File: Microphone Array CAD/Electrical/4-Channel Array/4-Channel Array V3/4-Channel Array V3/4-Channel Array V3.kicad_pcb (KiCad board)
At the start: 2 copper layers, 35 x 35 mm, 20 parts, among them J1 Conn_01x05_Pin, U1 74LCX125MTCX

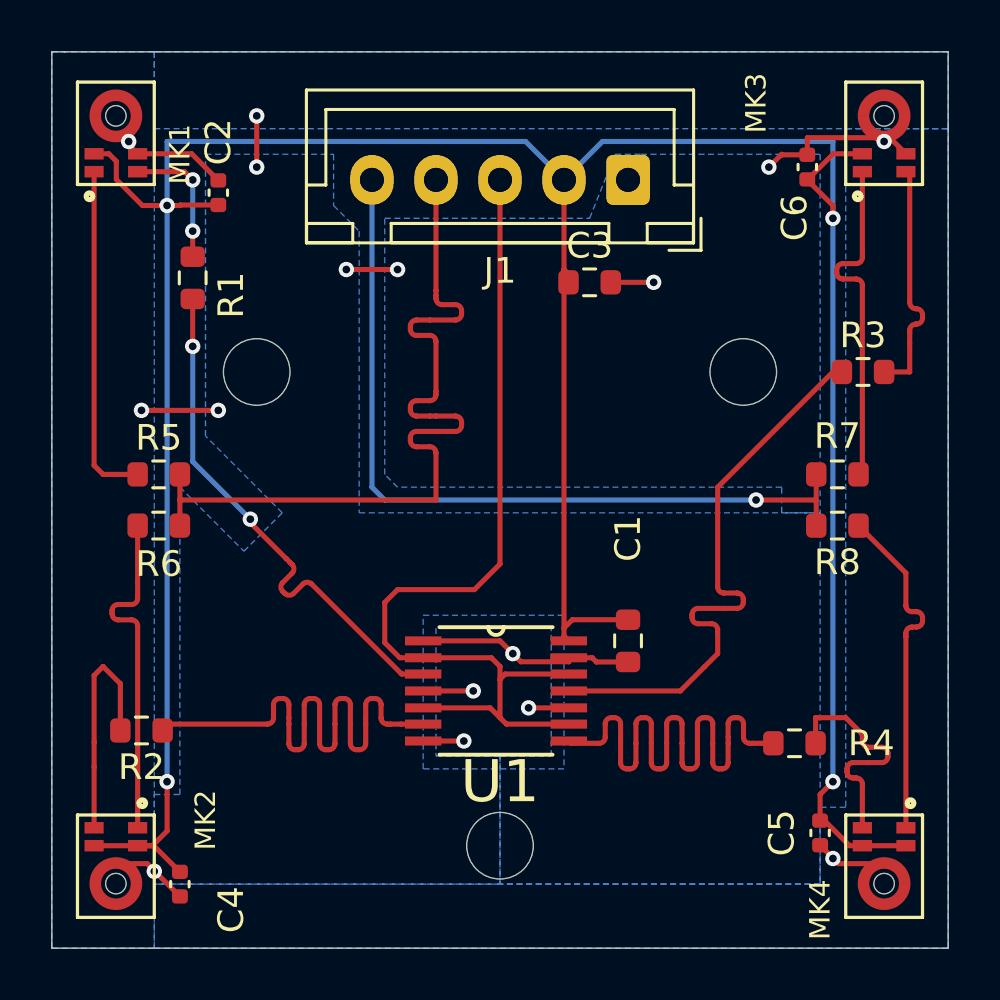
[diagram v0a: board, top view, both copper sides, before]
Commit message: Continued Array Development
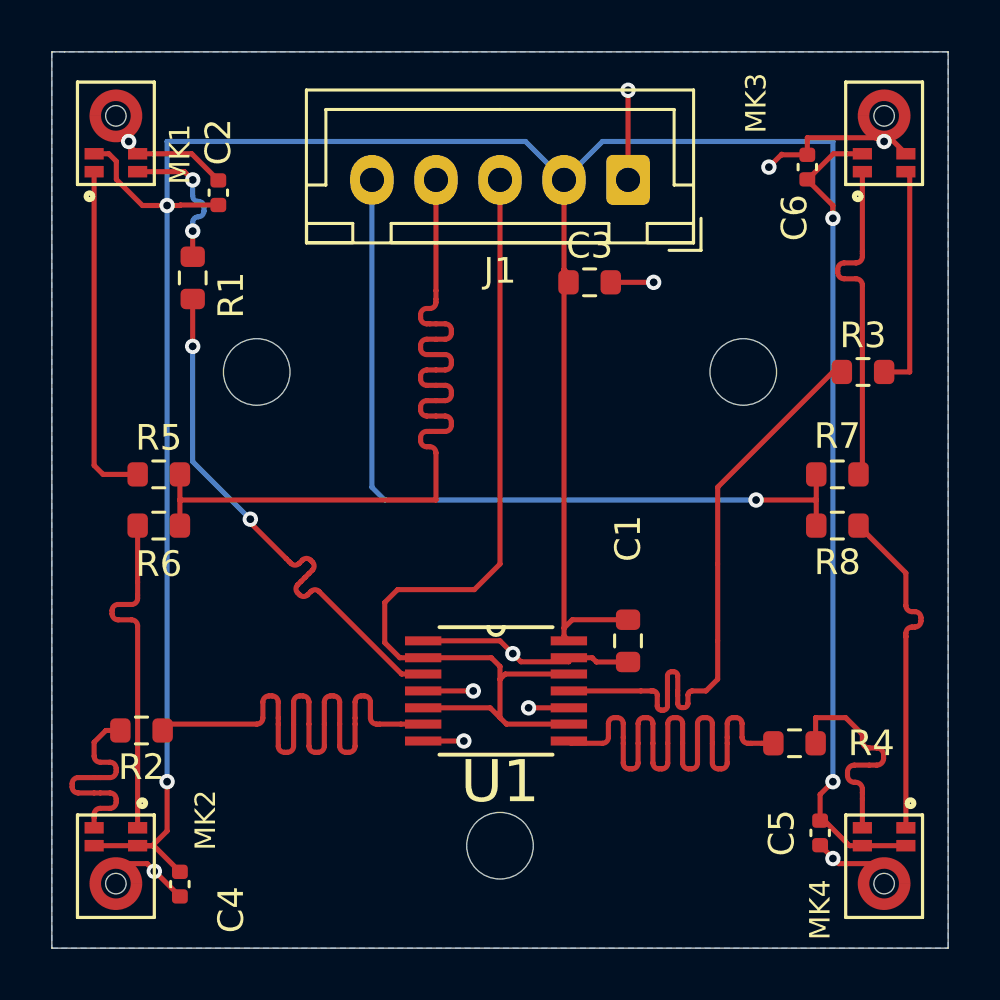
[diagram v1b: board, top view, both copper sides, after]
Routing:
- net Net-(J1-Pin_1): track 39.8 -> 36.3 mm, vias 16 -> 11
- net Net-(U1-O1): track 22.5 -> 23.9 mm
- net Net-(U1-O2): track 23.0 -> 23.9 mm
- net Net-(MK3-CLK): track 9.43 -> 8.88 mm

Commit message: Restructure
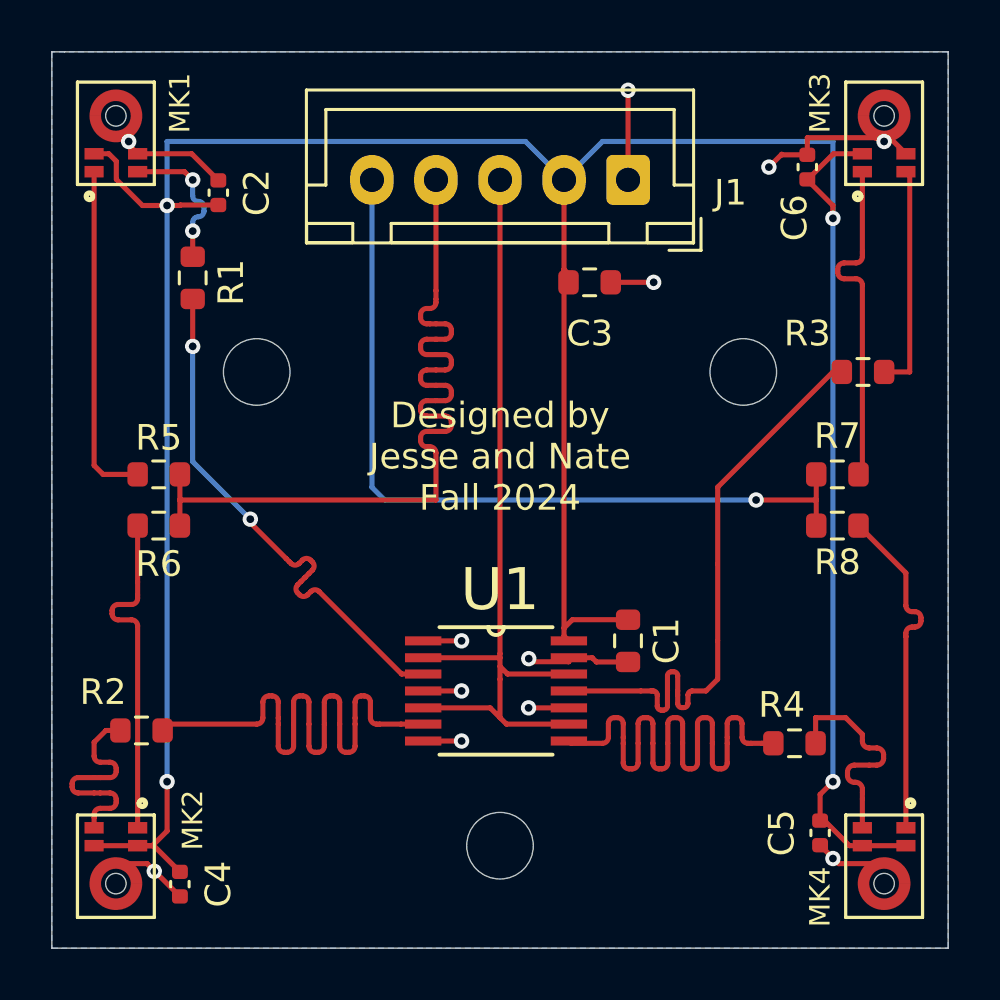
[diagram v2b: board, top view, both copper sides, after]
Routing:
- net Net-(J1-Pin_3): track 37.3 -> 32.8 mm
- net Net-(J1-Pin_1): track 36.3 -> 32.9 mm, vias 11 -> 12
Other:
- board text added: "Designed by Jesse and Nate Fall 2024"
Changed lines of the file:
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@@
 		(tags "connector JST XH vertical")
 		(property "Reference" "J1"
-			(at 5 -3.55 0)
+			(at -4 -0.5 0)
 			(layer "F.SilkS")
 			(effects
@@
 		(tags "resistor")
 		(property "Reference" "R3"
-			(at 0 -1.43 0)
+			(at -2.175 -1.5 0)
 			(layer "F.SilkS")
 			(effects
@@
 		(tags "resistor")
 		(property "Reference" "R1"
-			(at -0.675 1.5 90)
+			(at -0.175 1.5 90)
 			(layer "F.SilkS")
 			(effects
@@
 		(tags "capacitor")
 		(property "Reference" "C2"
-			(at 1.98 0 90)
+			(at 0 1.5 90)
 			(layer "F.SilkS")
 			(effects
@@
 		(tags "resistor")
 		(property "Reference" "C3"
-			(at 0 -1.43 0)
+			(at 0 2 0)
 			(layer "F.SilkS")
 			(effects
@@
 		(at 180 79.3 -90)
 		(property "Reference" "MK4"
-			(at 1.7 2.5 90)
+			(at 1.2 2.5 90)
 			(layer "F.SilkS")
 			(effects
@@
 		(at 150 79.3 -90)
 		(property "Reference" "MK2"
-			(at -1.8 -3.5 90)
+			(at -1.8 -3 90)
 			(layer "F.SilkS")
 			(effects
@@
 		(at 180 50.68 90)
 		(property "Reference" "MK3"
-			(at 1.18 -5 90)
+			(at 1.18 -2.5 90)
 			(layer "F.SilkS")
 			(effects
@@
 		(at 164.8448 72.4558)
 		(property "Reference" "U1"
-			(at 0.1552 3.5442 0)
+			(at 0.1552 -3.9558 0)
 			(layer "F.SilkS")
 			(effects
@@
 		(tags "resistor")
 		(property "Reference" "R2"
-			(at 0 -1.43 0)
+			(at 1.5 1.5 0)
 			(layer "F.SilkS")
 			(effects
@@
 		(tags "resistor")
 		(property "Reference" "C1"
-			(at 4 0 90)
+			(at 0 1.5 90)
 			(layer "F.SilkS")
 			(effects
@@
 		(tags "capacitor")
 		(property "Reference" "C4"
-			(at 1 -2 90)
+			(at 0 -1.5 90)
 			(layer "F.SilkS")
 			(effects
@@
 		(tags "resistor")
 		(property "Reference" "R4"
-			(at 3 0 0)
+			(at -0.5 -1.5 0)
 			(layer "F.SilkS")
 			(effects
@@
 		(at 150 50.68 90)
 		(property "Reference" "MK1"
-			(at -0.82 2.5 90)
+			(at 1.18 2.5 90)
 			(layer "F.SilkS")
 			(effects
@@
 		(layer "Edge.Cuts")
 	)
+	(gr_text "Designed by \nJesse and Nate\nFall 2024"
+		(at 165 65.5 0)
+		(layer "F.SilkS")
+		(effects
+			(font
+				(size 1 1)
+				(thickness 0.1)
+			)
+			(justify bottom)
+		)
+	)
 	(segment
 		(start 149.725 51.48)
@@
 	)
 	(segment
+		(start 166.1162 73.1162)
+		(end 167.6896 73.1162)
+		(width 0.2)
+		(layer "F.Cu")
+		(net 2)
+	)
+	(segment
 		(start 151.5 79.48)
 		(end 151.22 79.2)
@@
 	)
 	(segment
+		(start 163.5 72.4558)
+		(end 162 72.4558)
+		(width 0.2)
+		(layer "F.Cu")
+		(net 2)
+	)
+	(segment
 		(start 168.6008 71.1604)
 		(end 168.7654 71.325)
@@
 	)
 	(segment
-		(start 165.8176 71.3176)
-		(end 167.6824 71.3176)
-		(width 0.2)
-		(layer "F.Cu")
-		(net 2)
-	)
-	(segment
 		(start 151.22 79.2)
 		(end 150 79.2)
@@
 	)
 	(segment
-		(start 167.6824 71.3176)
-		(end 167.6896 71.3104)
-		(width 0.2)
-		(layer "F.Cu")
-		(net 2)
-	)
-	(segment
 		(start 152.96 51.48)
 		(end 150.85 51.48)
@@
 	)
 	(segment
-		(start 167.6896 71.3104)
-		(end 167.6896 71.1604)
+		(start 177 51.54)
+		(end 177 50.853333)
 		(width 0.2)
 		(layer "F.Cu")
@@
 	)
 	(segment
-		(start 177 51.54)
-		(end 177 50.853333)
+		(start 150 50.78)
+		(end 150.15 50.78)
 		(width 0.2)
 		(layer "F.Cu")
@@
 	)
 	(segment
-		(start 150 50.78)
-		(end 150.15 50.78)
+		(start 180 79.2)
+		(end 178.22 79.2)
 		(width 0.2)
 		(layer "F.Cu")
@@
 	)
 	(segment
-		(start 163.5884 74.4116)
-		(end 162 74.4116)
+		(start 170 52.5)
+		(end 170 49)
 		(width 0.2)
 		(layer "F.Cu")
@@
 	)
 	(segment
-		(start 162 70.5)
-		(end 165 70.5)
+		(start 150.5 51)
+		(end 150.5 51.13)
 		(width 0.2)
 		(layer "F.Cu")
@@
 	)
 	(segment
-		(start 165.5 71)
-		(end 165.8176 71.3176)
+		(start 166.1222 71.1954)
+		(end 166.2444 71.3176)
 		(width 0.2)
 		(layer "F.Cu")
@@
 	)
 	(segment
-		(start 180 79.2)
-		(end 178.22 79.2)
+		(start 180 50.78)
+		(end 180.15 50.78)
 		(width 0.2)
 		(layer "F.Cu")
@@
 	)
 	(segment
-		(start 170 52.5)
-		(end 170 49)
+		(start 167.6896 71.3104)
+		(end 167.6896 71.1604)
 		(width 0.2)
 		(layer "F.Cu")
@@
 	)
 	(segment
-		(start 150.5 51)
-		(end 150.5 51.13)
+		(start 163.5 74.4116)
+		(end 162 74.4116)
 		(width 0.2)
 		(layer "F.Cu")
@@
 	)
 	(segment
-		(start 180 50.78)
-		(end 180.15 50.78)
+		(start 178 78.98)
+		(end 177.5 78.48)
 		(width 0.2)
 		(layer "F.Cu")
@@
 	)
 	(segment
-		(start 163.9558 72.4558)
-		(end 162 72.4558)
+		(start 167.6824 71.3176)
+		(end 167.6896 71.3104)
 		(width 0.2)
 		(layer "F.Cu")
@@
 	)
 	(segment
-		(start 178 78.98)
-		(end 177.5 78.48)
+		(start 166.2444 71.3176)
+		(end 167.6824 71.3176)
 		(width 0.2)
 		(layer "F.Cu")
@@
 	)
 	(segment
-		(start 166.1162 73.1162)
-		(end 167.6896 73.1162)
+		(start 163.5 70.5)
+		(end 162 70.5)
 		(width 0.2)
 		(layer "F.Cu")
@@
 		(net 2)
 	)
-	(segment
-		(start 165 70.5)
-		(end 165.5 71)
-		(width 0.2)
-		(layer "F.Cu")
-		(net 2)
-	)
 	(via
 		(at 151.5 79.5)
@@
 	)
 	(via
-		(at 163.5884 74.4116)
+		(at 163.5 74.4116)
 		(size 0.6)
 		(drill 0.3)
@@
 	)
 	(via
-		(at 163.9558 72.4558)
+		(at 163.5 70.5)
 		(size 0.6)
 		(drill 0.3)
 		(layers "F.Cu" "B.Cu")
+		(free yes)
 		(net 2)
 	)
 	(via
-		(at 165.5 71)
+		(at 163.5 72.4558)
+		(size 0.6)
+		(drill 0.3)
+		(layers "F.Cu" "B.Cu")
+		(net 2)
+	)
+	(via
+		(at 166.1222 71.1954)
 		(size 0.6)
 		(drill 0.3)
@@
 	)
 	(segment
-		(start 165 67.5)
-		(end 164 68.5)
-		(width 0.2)
-		(layer "F.Cu")
-		(net 3)
-	)
-	(segment
-		(start 160.5 70.5716)
-		(end 161.0888 71.1604)
-		(width 0.2)
-		(layer "F.Cu")
-		(net 3)
-	)
-	(segment
-		(start 164 68.5)
-		(end 161 68.5)
+		(start 162 71.1604)
+		(end 165 71.1604)
 		(width 0.2)
 		(layer "F.Cu")
@@
 	)
 	(segment
-		(start 167.6896 71.7954)
-		(end 165.2046 71.7954)
-		(width 0.2)
-		(layer "F.Cu")
-		(net 3)
-	)
-	(segment
-		(start 161.0888 71.1604)
-		(end 162 71.1604)
+		(start 165.2954 71.7954)
+		(end 165 71.5)
 		(width 0.2)
 		(layer "F.Cu")
@@
 	)
 	(segment
-		(start 165 71.5)
-		(end 165 72)
+		(start 165 52.5)
+		(end 165 71)
 		(width 0.2)
 		(layer "F.Cu")
@@
 	)
 	(segment
-		(start 164.6604 71.1604)
-		(end 165 71.5)
-		(width 0.2)
-		(layer "F.Cu")
-		(net 3)
-	)
-	(segment
-		(start 161 68.5)
-		(end 160.5 69)
-		(width 0.2)
-		(layer "F.Cu")
-		(net 3)
-	)
-	(segment
-		(start 162 71.1604)
-		(end 164.6604 71.1604)
-		(width 0.2)
-		(layer "F.Cu")
-		(net 3)
-	)
-	(segment
 		(start 165 72)
 		(end 165 73.5)
@@
 	)
 	(segment
-		(start 165 52.5)
-		(end 165 67.5)
+		(start 167.6896 71.7954)
+		(end 165.2954 71.7954)
 		(width 0.2)
 		(layer "F.Cu")
@@
 	)
 	(segment
-		(start 165.2046 71.7954)
+		(start 165 71)
 		(end 165 72)
 		(width 0.2)
 		(layer "F.Cu")
-		(net 3)
-	)
-	(segment
-		(start 160.5 69)
-		(end 160.5 70.5716)
-		(width 0.2)
-		(layer "F.Cu")

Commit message: Added UHart Logo and Fab Files
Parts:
- added G***: LOGO, kicad libs:uhartacslogo3, B.Cu at (165.0, 67.5)
